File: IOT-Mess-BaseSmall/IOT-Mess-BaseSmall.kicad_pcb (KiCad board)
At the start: 2 copper layers, 32.2 x 84 mm, 21 parts, among them J1 ESP_P16 / ESP12, J10 Jumper_2, J11 Jumper_2, J12 Jumper_2, J13 Jumper_2, J14 Jumper_2, J15 Jumper_2, J16 Jumper_2, J17 Jumper_2, J18 Jumper_2, J19 Jumper_2, J2 ESP_P16 / C3, J20 Jumper_2, J21 Jumper_2, J3 ESP_P40, J4 Jumper_2, J5 Lolin32-Lite, J6 CH582, J7 Jumper_2, J8 Jumper_2, J9 Jumper_2

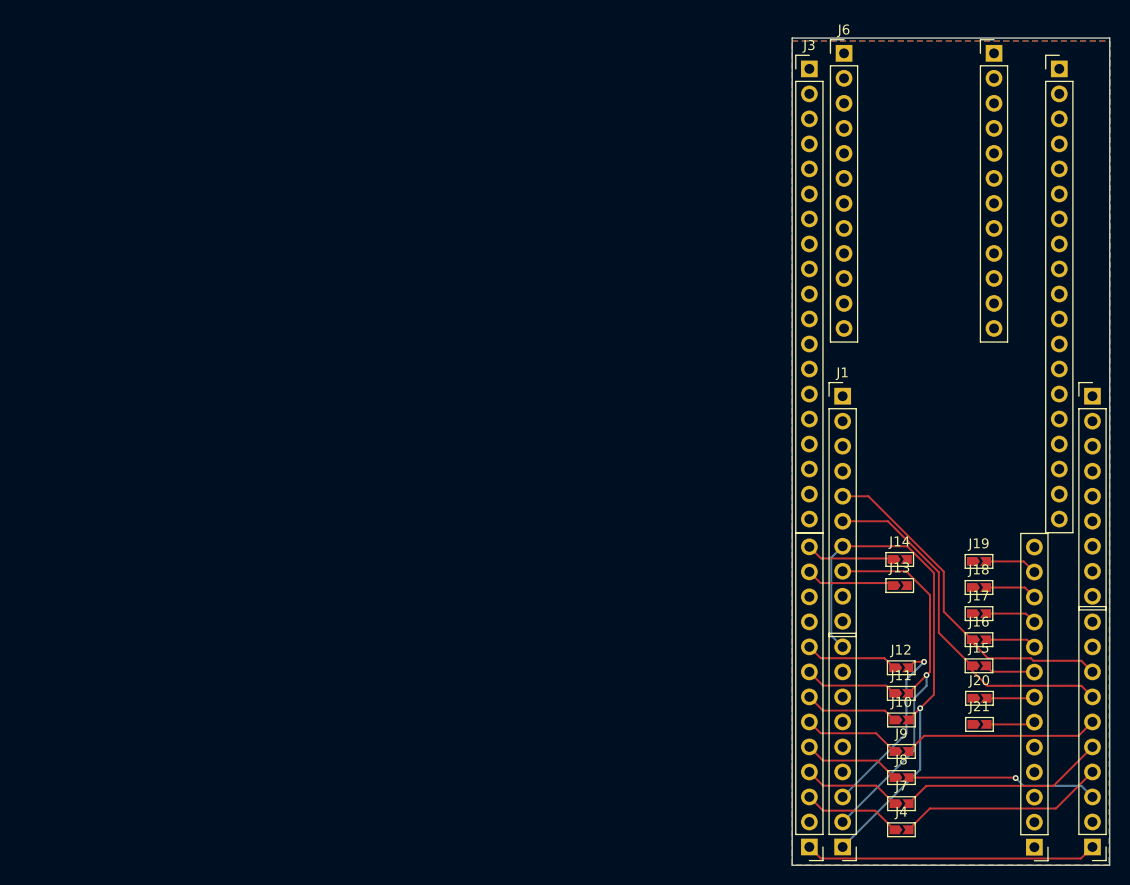
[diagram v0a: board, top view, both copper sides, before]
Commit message: did some works.
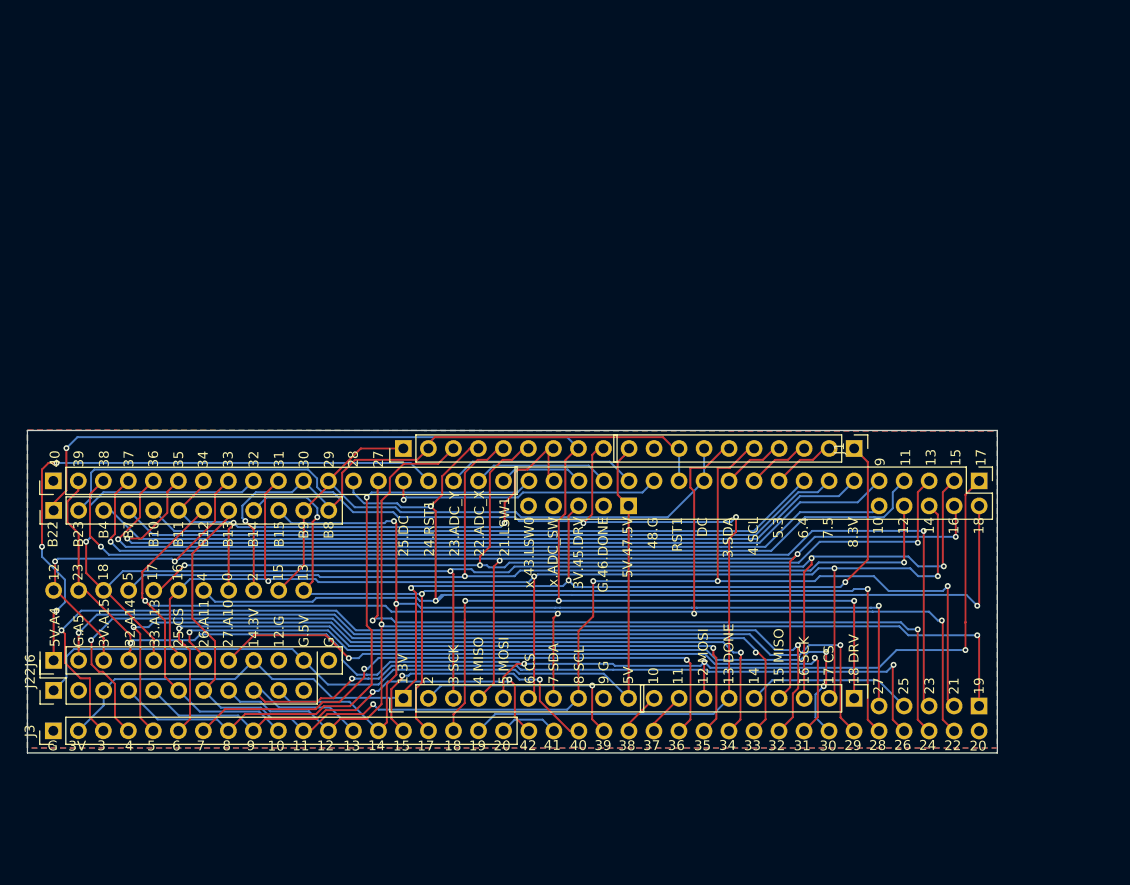
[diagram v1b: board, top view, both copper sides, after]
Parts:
- removed J10, J11, J12, J13, J14, J15, J16, J17, J18, J19, J20, J21, J4, J7, J8, J9: Jumper_2, IOT-Mess-Footprints:Jumpper-triangle
- removed J5: Lolin32-Lite, IOT-Mess-Footprints:Lolin32_Lite2
- added G***: LOGO, IOT-Mess-Footprints:catIcon8x8, B.Cu at (141.0, 100.0)
- added J22: Lolin32, IOT-Mess-Footprints:Lolin32-Adapter, F.Cu at (72.2, 112.1)
- added U1: ~, IOT-Mess-Footprints:CH_P48, F.Cu at (167.0, 90.0)
- moved J3 102.0 mm to (72.2, 116.2), turned to 90 degrees
- moved J6 101.2 mm to (72.2, 109.0), turned to 90 degrees
- moved J2 71.6 mm to (107.7, 112.9), turned to 90 degrees
- moved J1 5.44 mm to (153.5, 87.5), turned to -90 degrees
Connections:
- net CS_0 renamed CS
- net MISO_0 renamed MISO
- net MISO_1 renamed MISO2
- net MOSI_0 renamed MOSI
- net MOSI_1 renamed MOSI2
- net SCK_0 renamed SCK
- net SCL_0 renamed SCL
- net SDA_0 renamed SDA
- J1 pad P11: unconnected-(J1-Pin_13-PadP11) -> C37
- J1 pad P14: unconnected-(J1-Pin_16-PadP14) -> C25
- J1 pad P2: unconnected-(J1-Pin_2-PadP2) -> C5
- J1 pad P3: unconnected-(J1-Pin_3-PadP3) -> C4
- J1 pad P4: unconnected-(J1-Pin_4-PadP4) -> C3
- J2 pad P11: unconnected-(J2-Pin_13-PadP11) -> DRIVE
- J2 pad P12: unconnected-(J2-Pin_14-PadP12) -> ADC_SW
- J2 pad P13: unconnected-(J2-Pin_15-PadP13) -> LSW0
- J2 pad P14: unconnected-(J2-Pin_16-PadP14) -> LSW1
- J2 pad P15: unconnected-(J2-Pin_17-PadP15) -> ADC_X
- J2 pad P16: DRIVE -> ADC_Y
- J2 pad P2: unconnected-(J2-Pin_2-PadP2) -> C39
- J3 pad P12: unconnected-(J3-Pin_12-PadP12) -> ADC_Y
- J3 pad P13: SCK_1 -> SCK2
- J3 pad P15: unconnected-(J3-Pin_15-PadP15) -> C40
- J3 pad P18: unconnected-(J3-Pin_17-PadP18) -> DRIVE
- J3 pad P19: unconnected-(J3-Pin_18-PadP19) -> DONE
- J3 pad P20: unconnected-(J3-Pin_19-PadP20) -> C41
- J3 pad P21: unconnected-(J3-Pin_38-PadP21) -> C45
- J3 pad P22: unconnected-(J3-Pin_37-PadP22) -> C46
- J3 pad P23: unconnected-(J3-Pin_36-PadP23) -> C47
- J3 pad P25: unconnected-(J3-Pin_34-PadP25) -> C48
- J3 pad P27: unconnected-(J3-Pin_33-PadP27) -> C24
- J3 pad P28: unconnected-(J3-Pin_32-PadP28) -> ADC_X
- J3 pad P29: RST1 -> DC
- J3 pad P3: unconnected-(J3-Pin_3-PadP3) -> C32
- J3 pad P30: DC -> RST1
- J3 pad P34: unconnected-(J3-Pin_26-PadP34) -> ADC_SW
- J3 pad P35: unconnected-(J3-Pin_25-PadP35) -> C9
- J3 pad P36: unconnected-(J3-Pin_24-PadP36) -> C10
- J3 pad P37: unconnected-(J3-Pin_23-PadP37) -> C11
- J3 pad P38: unconnected-(J3-Pin_22-PadP38) -> C23
- J3 pad P4: unconnected-(J3-Pin_4-PadP4) -> C33
- J3 pad P5: unconnected-(J3-Pin_5-PadP5) -> C34
- J3 pad P6: unconnected-(J3-Pin_6-PadP6) -> C35
- J3 pad P7: unconnected-(J3-Pin_7-PadP7) -> C36
- J3 pad P8: SDA_1 -> SDA2
- J3 pad P9: SCL_1 -> SCL2
- J6 pad A10: unconnected-(J6-Pin_8-PadA10) -> C31
- J6 pad A11: unconnected-(J6-Pin_7-PadA11) -> C30
- J6 pad A5: unconnected-(J6-Pin_2-PadA5) -> C29
- J6 pad B10: unconnected-(J6-Pin_17-PadB10) -> C6
- J6 pad B11: unconnected-(J6-Pin_18-PadB11) -> ADC_SW
- J6 pad B4: unconnected-(J6-Pin_15-PadB4) -> C8
- J6 pad B7: unconnected-(J6-Pin_16-PadB7) -> C7
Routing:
- net SCK: track 19.5 -> 160.6 mm, vias 1 -> 4
- net MISO: track 21.1 -> 149.4 mm, vias 0 -> 5
- net DONE: track 0.00 -> 126.7 mm, vias 0 -> 2
- net DRIVE: track 19.0 -> 139.0 mm, vias 1 -> 4
- net ADC_X: track 0.00 -> 119.4 mm, vias 0 -> 3
- net SDA: track 36.6 -> 156.0 mm, vias 0 -> 4
- net ADC_Y: track 0.00 -> 117.6 mm, vias 0 -> 2
- net MOSI: track 21.1 -> 137.5 mm, vias 0 -> 4
- net CS: track 19.9 -> 131.3 mm, vias 0 -> 4
- net C23: track 0.00 -> 110.6 mm, vias 0 -> 2
- net MISO2: track 0.00 -> 105.9 mm, vias 0 -> 3
- net SCL: track 35.3 -> 140.3 mm, vias 0 -> 4
- net MOSI2: track 0.00 -> 103.6 mm, vias 0 -> 3
- net LSW0: track 0.00 -> 100.9 mm, vias 0 -> 3
- net LSW1: track 0.00 -> 100.8 mm, vias 0 -> 2
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- added copper zone on B.Cu, net GND
- added copper zone on F.Cu, net GND
- removed copper zone on B.Cu, net unconnected-(J2-Pin_2-PadP2)
- removed copper zone on F.Cu, net unconnected-(J2-Pin_2-PadP2)
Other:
- board size 32.2 x 84 mm -> 98.5 x 32.8 mm
- board text added: "0"
- board text added: "1 3V"
- board text added: "10"
- board text added: "11"
- board text added: "12"
- board text added: "12 MOSI"
- board text added: "12.G"
- board text added: "13"
- board text added: "13 DONE"
- board text added: "14"
- board text added: "14.3V"
- board text added: "15"
- board text added: "15 MISO"
- board text added: "16"
- board text added: "16 SCK"
- board text added: "17"
- board text added: "17 CS"
- board text added: "18"
- board text added: "18 DRV"
- board text added: "19"
- board text added: "2"
- board text added: "20"
- board text added: "21"
- board text added: "21.LSW1"
- board text added: "22"
- board text added: "22.ADC_X"
- board text added: "23"
- board text added: "23.ADC_Y"
- board text added: "24"
- board text added: "24.RST1"
- board text added: "25"
- board text added: "25.CS"
- board text added: "25.DC"
- board text added: "26"
- board text added: "26.A11"
- board text added: "27"
- board text added: "27.A10"
- board text added: "28"
- board text added: "29"
- board text added: "3"
- board text added: "3 SCK"
- board text added: "3.SDA"
- board text added: "30"
- board text added: "31"
- board text added: "32"
- board text added: "32.A14"
- board text added: "33"
- board text added: "33.A13"
- board text added: "34"
- board text added: "35"
- board text added: "36"
- board text added: "37"
- board text added: "38"
- board text added: "39"
- board text added: "3V"
- board text added: "3V.45.DRV"
- board text added: "3V.A15"
- board text added: "4"
- board text added: "4 MISO"
- board text added: "4.SCL"
- board text added: "40"
- board text added: "41"
- board text added: "42"
- board text added: "48.G"
- board text added: "5"
- board text added: "5 MOSI"
- board text added: "5.3"
- board text added: "5V"
- board text added: "5V.47.5V"
- board text added: "5V.A4"
- board text added: "6"
- board text added: "6 CS"
- board text added: "6.4"
- board text added: "7"
- board text added: "7 SDA"
- board text added: "7.5"
- board text added: "8"
- board text added: "8 SCL"
- board text added: "8.3V"
- board text added: "9"
- board text added: "9 G"
- board text added: "B10"
- board text added: "B11"
- board text added: "B12"
- board text added: "B13"
- board text added: "B14"
- board text added: "B15"
- board text added: "B22"
- board text added: "B23"
- board text added: "B4"
- board text added: "B7"
- board text added: "B8"
- board text added: "B9"
- board text added: "DC"
- board text added: "G"
- board text added: "G.46.DONE"
- board text added: "G.5V"
- board text added: "G.A5"
- board text added: "IOT_Mess AdapterB V1.0 07/05/25"
- board text added: "RST1"
- board text added: "x.43.LSW0"
- board text added: "x.ADC_SW"
